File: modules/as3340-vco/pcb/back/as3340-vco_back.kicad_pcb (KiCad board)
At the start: 2 copper layers, 37.8 x 70.2 mm, 35 parts, among them J1 IDC Header 2x8, J2 Pin Socket 1x9, U1 AS3340, U2 L79L05_TO92

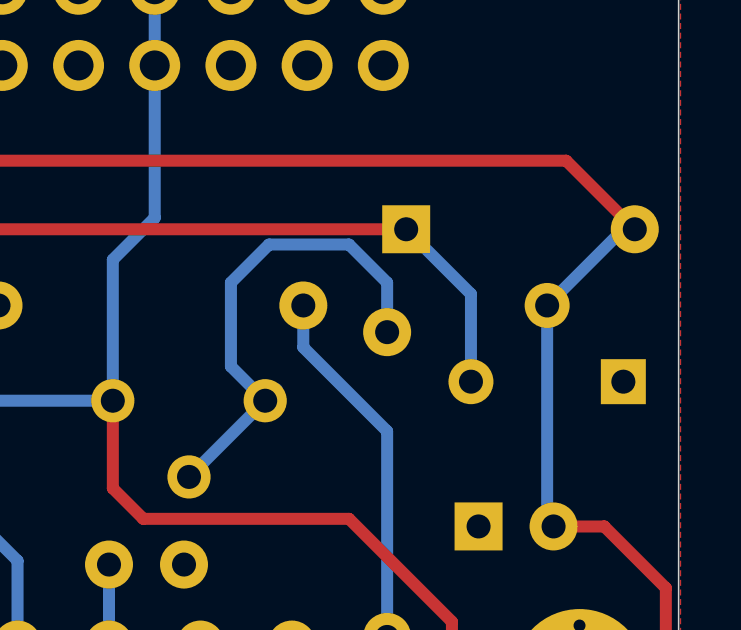
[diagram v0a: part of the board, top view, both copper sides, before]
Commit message: modules: as3340-vco: back: remove unconnected nets
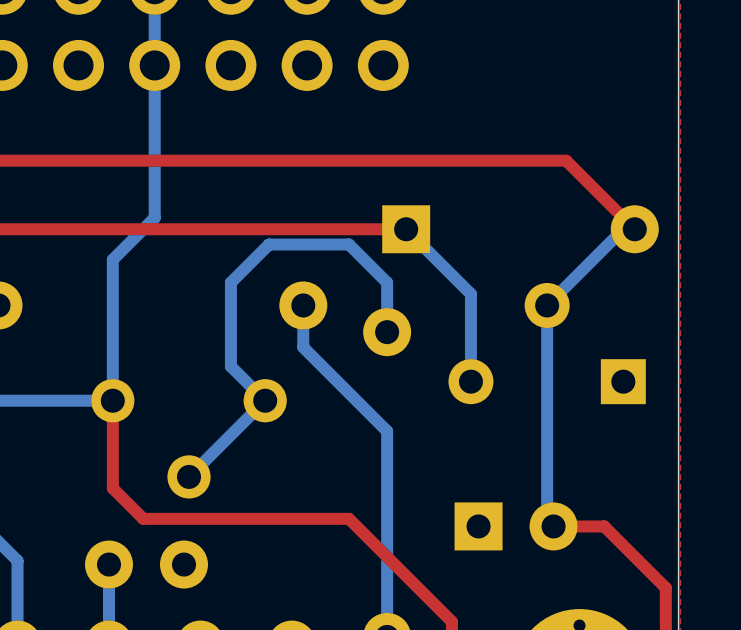
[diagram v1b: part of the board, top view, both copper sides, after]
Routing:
- net Net-(R9-Pad1): track 16.5 -> 15.9 mm
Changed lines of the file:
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@@
   (segment (start 161.163 90.932) (end 159.472 90.932) (width 0.4) (layer "F.Cu") (net 3))
   (segment (start 163.21449 92.98349) (end 161.163 90.932) (width 0.4) (layer "F.Cu") (net 3))
-  (segment (start 162.179 81.026) (end 161.798 81.026) (width 0.4) (layer "F.Cu") (net 3))
   (segment (start 163.21449 116.05851) (end 163.21449 92.98349) (width 0.4) (layer "F.Cu") (net 3))
   (segment (start 158.75 118.364) (end 160.909 118.364) (width 0.4) (layer "F.Cu") (net 3))
@@
   (segment (start 133.604 104.394) (end 135.255 104.394) (width 0.4) (layer "B.Cu") (net 14))
   (segment (start 140.97 83.566) (end 138.176 83.566) (width 0.4) (layer "B.Cu") (net 15))
-  (segment (start 132.842 94.488) (end 132.842 94.488) (width 0.4) (layer "F.Cu") (net 16))
+  (segment (start 132.334 81.026) (end 130.643 82.717) (width 0.4) (layer "F.Cu") (net 16))
+  (segment (start 145.669 114.427) (end 145.669 115.824) (width 0.4) (layer "F.Cu") (net 16))
   (segment (start 144.145 112.903) (end 145.669 114.427) (width 0.4) (layer "F.Cu") (net 16))
-  (segment (start 132.334 81.026) (end 130.643 82.717) (width 0.4) (layer "F.Cu") (net 16))
+  (segment (start 130.643 82.717) (end 130.643 83.439) (width 0.4) (layer "F.Cu") (net 16))
   (segment (start 133.223 112.903) (end 144.145 112.903) (width 0.4) (layer "F.Cu") (net 16))
-  (segment (start 130.643 82.717) (end 130.643 83.439) (width 0.4) (layer "F.Cu") (net 16))
-  (segment (start 145.669 114.427) (end 145.669 115.824) (width 0.4) (layer "F.Cu") (net 16))
   (segment (start 130.683 110.363) (end 133.223 112.903) (width 0.4) (layer "F.Cu") (net 16))
+  (segment (start 132.842 100.965) (end 130.683 103.124) (width 0.4) (layer "F.Cu") (net 16))
   (segment (start 132.842 94.488) (end 132.842 100.965) (width 0.4) (layer "F.Cu") (net 16))
-  (segment (start 132.842 100.965) (end 130.683 103.124) (width 0.4) (layer "F.Cu") (net 16))
+  (segment (start 130.683 103.124) (end 130.683 110.363) (width 0.4) (layer "F.Cu") (net 16))
   (segment (start 154.559 81.026) (end 132.334 81.026) (width 0.4) (layer "F.Cu") (net 16))
-  (segment (start 130.683 103.124) (end 130.683 110.363) (width 0.4) (layer "F.Cu") (net 16))
   (via (at 132.842 94.488) (size 0.8) (drill 0.4) (layers "F.Cu" "B.Cu") (net 16))
   (segment (start 156.163 129.239) (end 154.098 127.174) (width 0.4) (layer "B.Cu") (net 16))
-  (segment (start 132.842 85.638) (end 130.643 83.439) (width 0.4) (layer "B.Cu") (net 16))
   (segment (start 144.653 122.555) (end 147.701 125.603) (width 0.4) (layer "B.Cu") (net 16))
   (segment (start 156.718 86.106) (end 156.718 83.185) (width 0.4) (layer "B.Cu") (net 16))
@@
   (segment (start 156.718 83.185) (end 154.559 81.026) (width 0.4) (layer "B.Cu") (net 16))
   (segment (start 149.526 127.174) (end 147.701 128.999) (width 0.4) (layer "B.Cu") (net 16))
-  (segment (start 132.842 94.488) (end 132.842 85.638) (width 0.4) (layer "B.Cu") (net 16))
   (segment (start 147.701 128.999) (end 147.701 129.159) (width 0.4) (layer "B.Cu") (net 16))
   (segment (start 145.669 115.824) (end 145.669 117.983) (width 0.4) (layer "B.Cu") (net 16))
+  (segment (start 132.842 85.638) (end 130.643 83.439) (width 0.4) (layer "B.Cu") (net 16))
+  (segment (start 132.842 94.488) (end 132.842 85.638) (width 0.4) (layer "B.Cu") (net 16))
   (segment (start 154.098 127.174) (end 149.526 127.174) (width 0.4) (layer "B.Cu") (net 16))
   (segment (start 145.669 117.983) (end 144.653 118.999) (width 0.4) (layer "B.Cu") (net 16))
@@
   (segment (start 148.717 82.804) (end 148.717 85.598) (width 0.4) (layer "B.Cu") (net 22))
   (segment (start 148.717 85.598) (end 149.86 86.741) (width 0.4) (layer "B.Cu") (net 22))
-  (segment (start 150.241 86.36) (end 149.86 86.741) (width 0.4) (layer "B.Cu") (net 22))
   (segment (start 149.86 86.741) (end 147.32 89.281) (width 0.4) (layer "B.Cu") (net 22))
   (segment (start 153.924 82.804) (end 152.654 81.534) (width 0.4) (layer "B.Cu") (net 22))
